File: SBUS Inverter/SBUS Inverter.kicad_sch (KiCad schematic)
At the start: 2 parts, among them Q1 2N2222

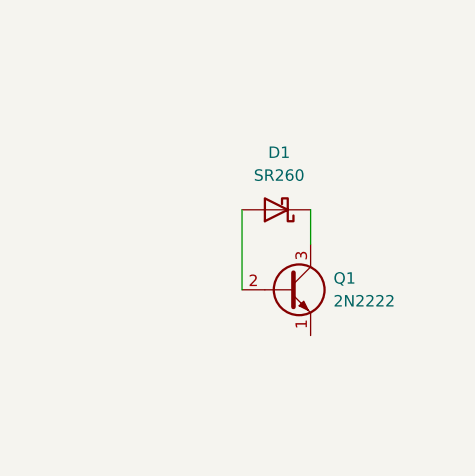
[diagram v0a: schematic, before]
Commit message: Finishing up the SBUS inverter.
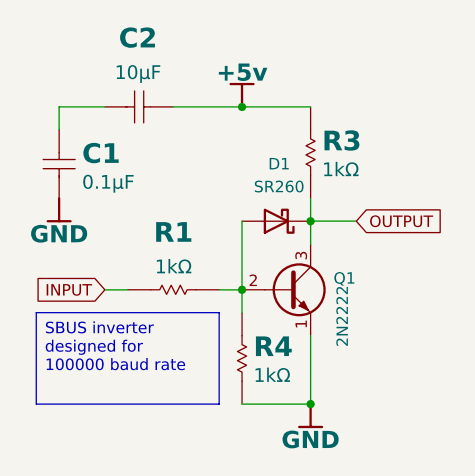
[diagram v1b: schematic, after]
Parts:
- added C1: 0.1µF, wavenumber:C1812_MD, symbol wn__wavenumber:C_2P_NP
- added C2: 10µF, wavenumber:C0603_0.90MM_MD, symbol wn__wavenumber:C_2P_NP
- added R1, R3, R4: 1kΩ, wavenumber:R2010_0.70MM_MD, symbol wn__wavenumber:R_2P
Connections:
- net GND: now reaches Q1.1 (E)
- net GND: now also C1.2 (1), R4.1
- net at D1.2 (A), Q1.2 (B): now also R1.2, R4.2
- net OUTPUT: now reaches D1.1 (K), Q1.3 (C)
- net OUTPUT: now also R3.1
- new net: C1.1, C2.2 (1)
- new net +5v: C2.1, R3.2
- new net INPUT: R1.1
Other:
- moved on the sheet: D1

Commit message: Improving the circuit.
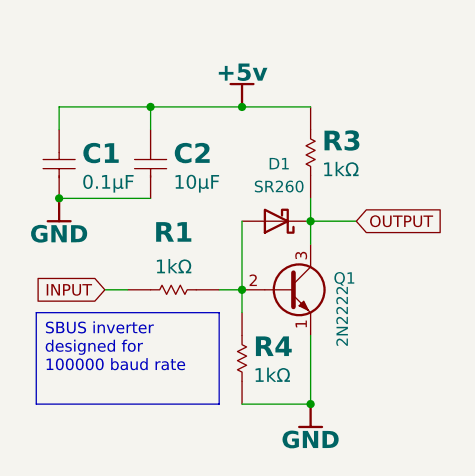
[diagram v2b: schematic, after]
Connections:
- net +5v: now also C1.1
- net GND: now also C2.2 (1)
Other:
- moved on the sheet: C2
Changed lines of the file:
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@@
+	)
+	(junction
+		(at 116.84 66.04)
+		(diameter 0)
+		(color 0 0 0 0)
 	)
 	(junction
@@
 	)
 	(junction
+		(at 106.68 76.2)
+		(diameter 0)
+		(color 0 0 0 0)
+	)
+	(junction
 		(at 127 66.04)
 		(diameter 0)
@@
 	(wire
 		(pts
+			(xy 106.68 66.04) (xy 116.84 66.04)
+		)
+		(stroke
+			(width 0)
+			(type default)
+		)
+	)
+	(wire
+		(pts
 			(xy 124.46 86.36) (xy 127 86.36)
 		)
@@
 	(wire
 		(pts
-			(xy 111.76 66.04) (xy 106.68 66.04)
-		)
-		(stroke
-			(width 0)
-			(type default)
-		)
-	)
-	(wire
-		(pts
 			(xy 134.62 78.74) (xy 134.62 81.28)
 		)
@@
 	(wire
 		(pts
-			(xy 119.38 66.04) (xy 127 66.04)
-		)
-		(stroke
-			(width 0)
-			(type default)
-		)
-	)
-	(wire
-		(pts
 			(xy 127 66.04) (xy 134.62 66.04)
 		)
@@
 	(wire
 		(pts
+			(xy 106.68 76.2) (xy 116.84 76.2)
+		)
+		(stroke
+			(width 0)
+			(type default)
+		)
+	)
+	(wire
+		(pts
 			(xy 111.76 86.36) (xy 114.3 86.36)
 		)
@@
 	(wire
 		(pts
+			(xy 116.84 66.04) (xy 127 66.04)
+		)
+		(stroke
+			(width 0)
+			(type default)
+		)
+	)
+	(wire
+		(pts
 			(xy 127 99.06) (xy 134.62 99.06)
+		)
+		(stroke
+			(width 0)
+			(type default)
+		)
+	)
+	(wire
+		(pts
+			(xy 116.84 66.04) (xy 116.84 68.58)
 		)
 		(stroke
@@
 		(lib_name "C_2P_NP_1")
 		(lib_id "wn__wavenumber:C_2P_NP")
-		(at 119.38 66.04 180)
+		(at 116.84 68.58 270)
 		(unit 1)
 		(exclude_from_sim no)
@@
 		(fields_autoplaced yes)
 		(property "Reference" "C2"
-			(at 115.443 58.42 0)
+			(at 119.38 71.247 90)
 			(effects
 				(font
@@
 					(bold yes)
 				)
+				(justify left)
 			)
 		)
 		(property "Value" "10µF"
-			(at 115.443 62.23 0)
+			(at 119.38 74.422 90)
 			(effects
 				(font
@@
 					(thickness 0.15)
 				)
+				(justify left)
 			)
 		)
 		(property "Footprint" "wavenumber:C0603_0.90MM_MD"
-			(at 119.38 66.04 0)
+			(at 116.84 68.58 0)
 			(effects
 				(font
@@
 		)
 		(property "Datasheet" ""
-			(at 119.38 66.04 0)
+			(at 116.84 68.58 0)
 			(effects
 				(font
@@
 		)
 		(property "Description" ""
-			(at 119.38 66.04 0)
+			(at 116.84 68.58 0)
 			(effects
 				(font
@@
 		)
 		(property "Internal Part Number" ""
-			(at 119.38 66.04 0)
+			(at 116.84 68.58 0)
 			(effects
 				(font
@@
 		)
 		(property "Manufacturer" "Murata Electronics"
-			(at 119.38 66.04 0)
+			(at 116.84 68.58 0)
 			(effects
 				(font
@@
 		)
 		(property "Manufacturer Part Number" "GRT188R61E106ME13D"
-			(at 119.38 66.04 0)
+			(at 116.84 68.58 0)
 			(effects
 				(font
@@
 		)
 		(property "cad-reference" "GRT188R61E106ME13D"
-			(at 119.38 66.04 0)
+			(at 116.84 68.58 0)
 			(effects
 				(font
@@
 		)
 		(property "flags" ""
-			(at 119.38 66.04 0)
-			(effects
-				(font
+			(at 116.84 68.58 0)
+			(effects
+				(font
